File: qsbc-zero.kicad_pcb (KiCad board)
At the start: 4 copper layers, 80 x 80 mm, 242 parts, among them J1 Micro_SD_Card_Det1, J10 Conn_02x18_Odd_Even, J11 Conn_01x09_Male, J2 USB4105, J3 USB-A-S-F-B-VU, J4 USB4105, J5 Conn_02x18_Odd_Even, J6 J1B1211CCD, J7 Conn_01x06_Male, J8 Conn_01x09_Male, J9 Conn_01x02_Male, SW1 SW_Push, U1 MX6UL-VM, U11 TPD4EUSB30, U12 74LVC1G04, U13 D5V0H1B2LP, U14 D5V0H1B2LP, U18 DP83825, U2 MC32PF1510A6EP, U25 TPD4EUSB30, U26 TPD4EUSB30, U27 TPD4EUSB30, U3 MT41K256M16, U4 TUSB320, U5 AP22811B, U6 TPD4EUSB30, U7 D5V0H1B2LP, U8 D5V0H1B2LP, U9 W25Q512JVEIQ, Y1 24Mhz, Y2 32.768kHz

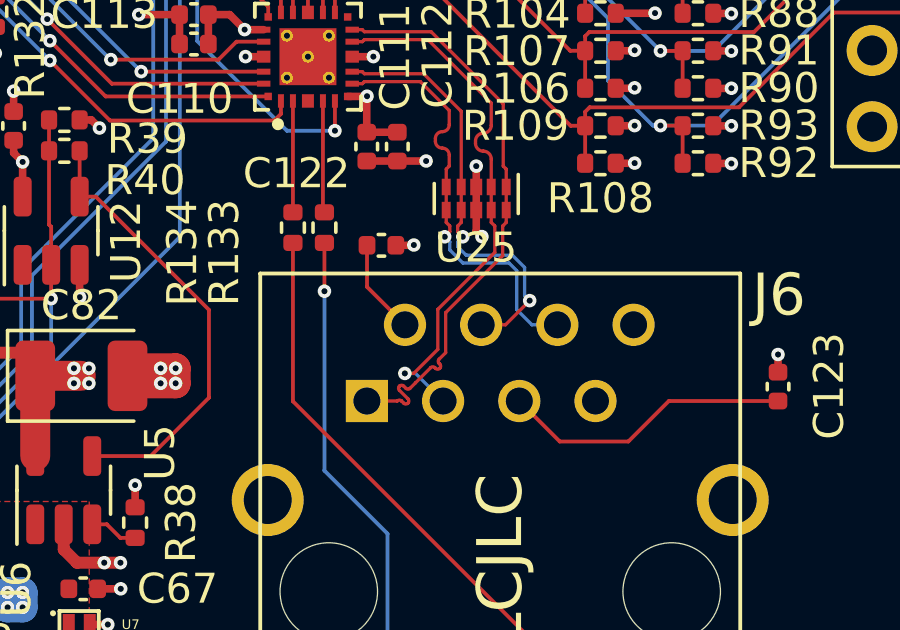
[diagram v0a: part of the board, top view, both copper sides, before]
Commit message: misc fixes, add pics of board
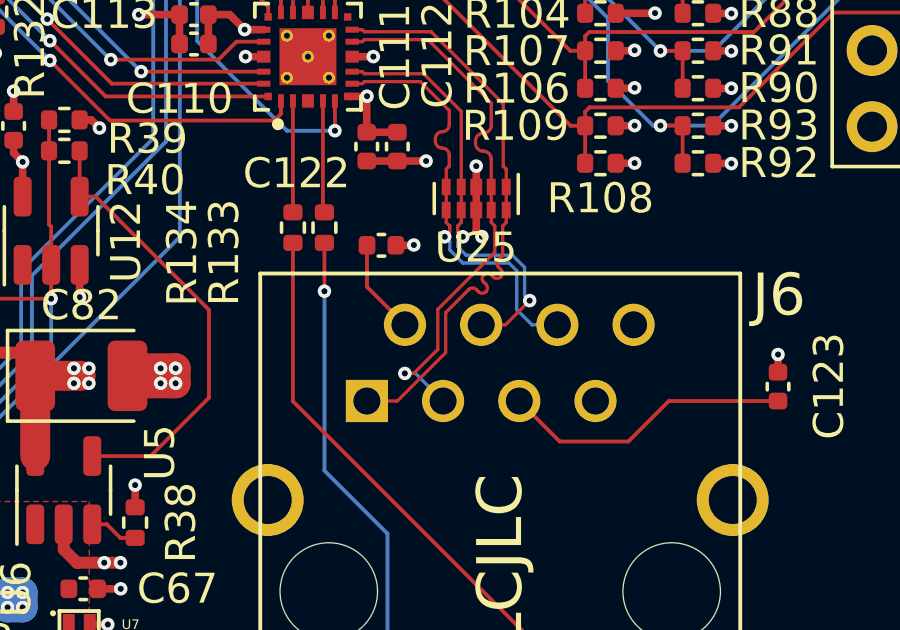
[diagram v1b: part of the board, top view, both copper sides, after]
